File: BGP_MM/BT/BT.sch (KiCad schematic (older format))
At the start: 26 parts, among them J1 Conn_01x02_Male, J2 Conn_01x05_Male, U1 TS512A

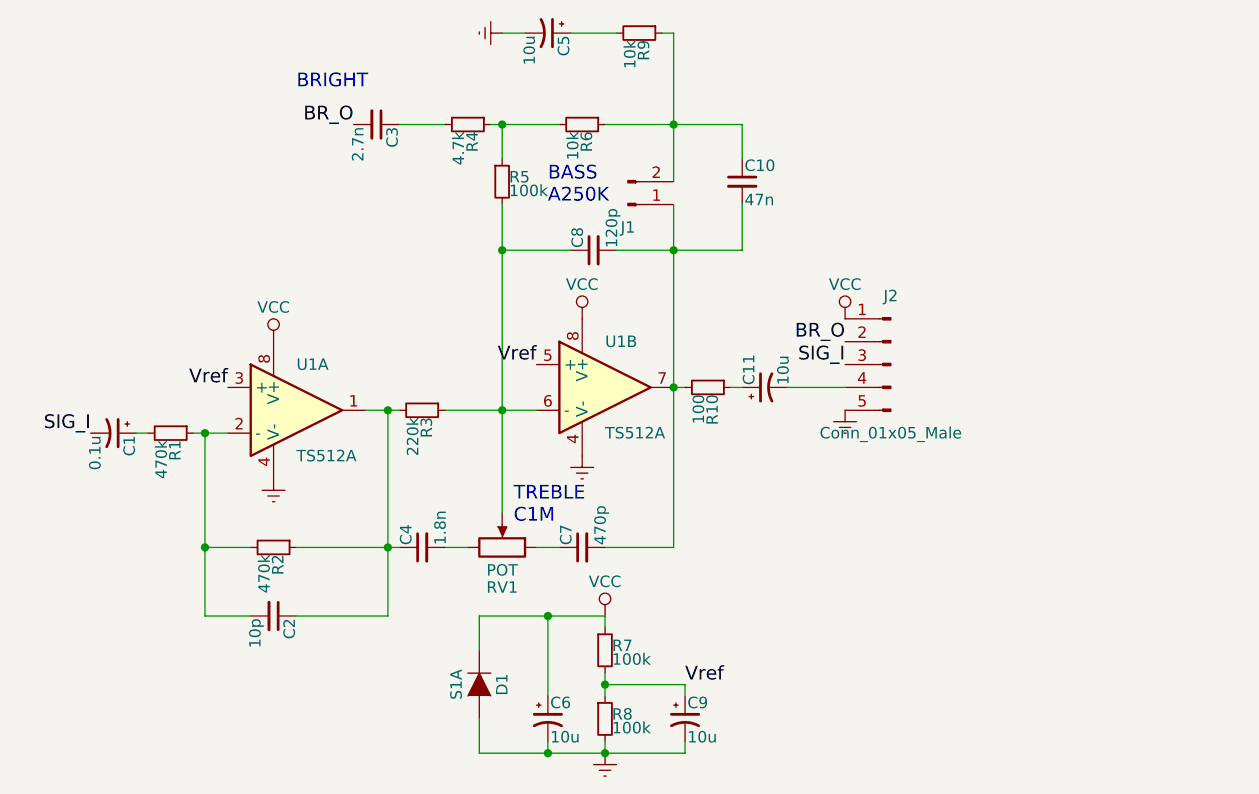
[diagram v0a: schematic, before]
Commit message: MM Gerbers
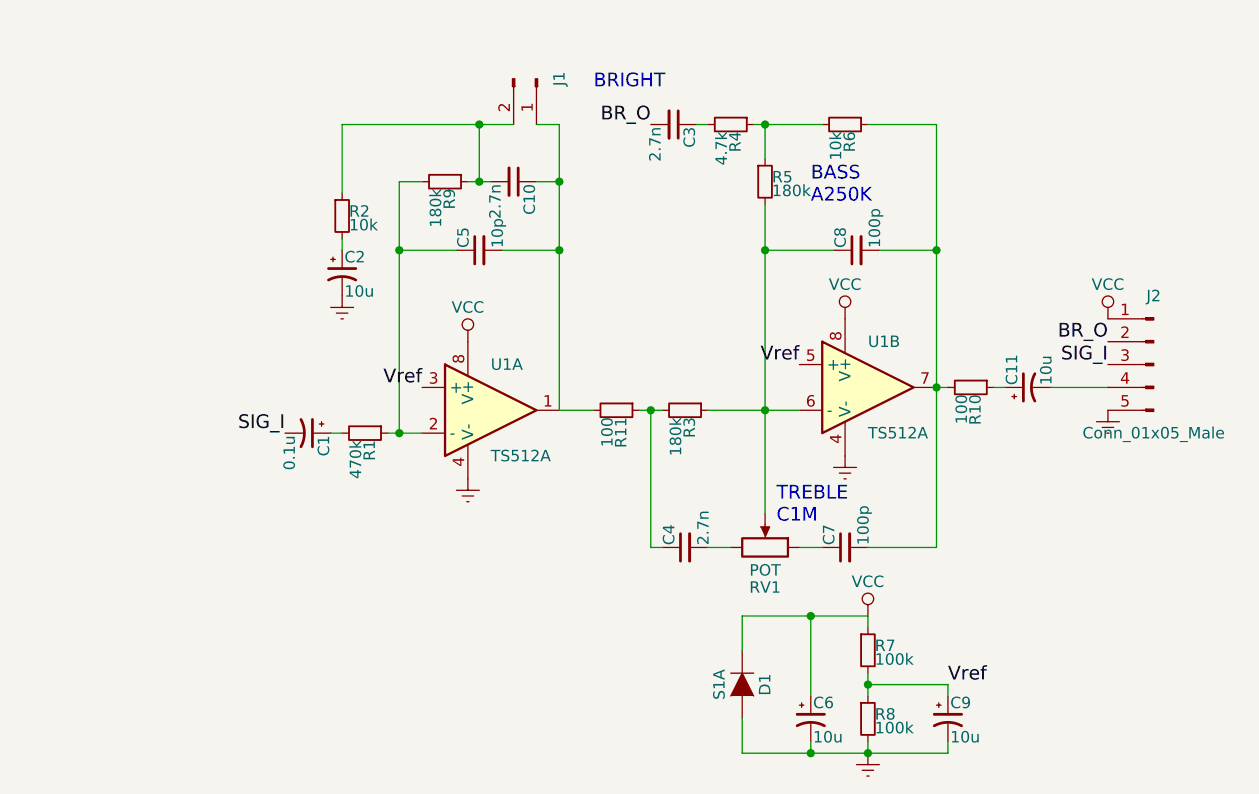
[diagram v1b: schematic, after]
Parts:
- removed C2: 10p, Capacitors_SMD:C_0603_HandSoldering, symbol C_Small
- removed C5: 10u, Capacitors_SMD:C_0805, symbol CP1_Small
- added C2: 10u, Capacitors_SMD:C_0805, symbol CP1_Small
- added C5: 10p, Capacitors_SMD:C_0603_HandSoldering, symbol C_Small
- added R11: 100, Capacitors_SMD:C_0603_HandSoldering, symbol R_Small
- C10: value 47n -> 2.7n; footprint Capacitors_SMD:C_1206 -> Capacitors_SMD:C_0805
- C4: value 1.8n -> 2.7n
- C7: value 470p -> 100p
- C8: value 120p -> 100p
- J1: footprint Connectors_JST:JST_PH_B2B-PH-K_02x2.00mm_Straight -> Pin_Headers:Pin_Header_Straight_1x02
- R2: value 470k -> 10k
- R3: value 220k -> 180k
- R5: value 100k -> 180k
- R9: value 10k -> 180k
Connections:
- net Earth: now also C2.2
- net at C4.1, R3.2: now also R11.1; no longer R2.1, U1.1
- net at C7.2, C8.2, R10.2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: now also R6.1; no longer C10.2, J1.1 (Pin_1)
- net at J1.2 (Pin_2), R9.1: now also C10.2, R2.1; no longer C10.1, R6.1
- net at R9.2: now also R1.1, U1.2 (-), C5.1
- new net: C10.1, C5.2, J1.1 (Pin_1), R11.2, U1.1
- new net: C2.1, R2.2
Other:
- moved on the sheet: C1, C11, C3, C4, C6, C7, C8, C9, D1, J2, R1, R10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
